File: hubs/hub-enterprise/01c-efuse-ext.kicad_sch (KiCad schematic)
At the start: 12 parts, among them J103 PJ-002AH, U103 TPS25940LRVCR

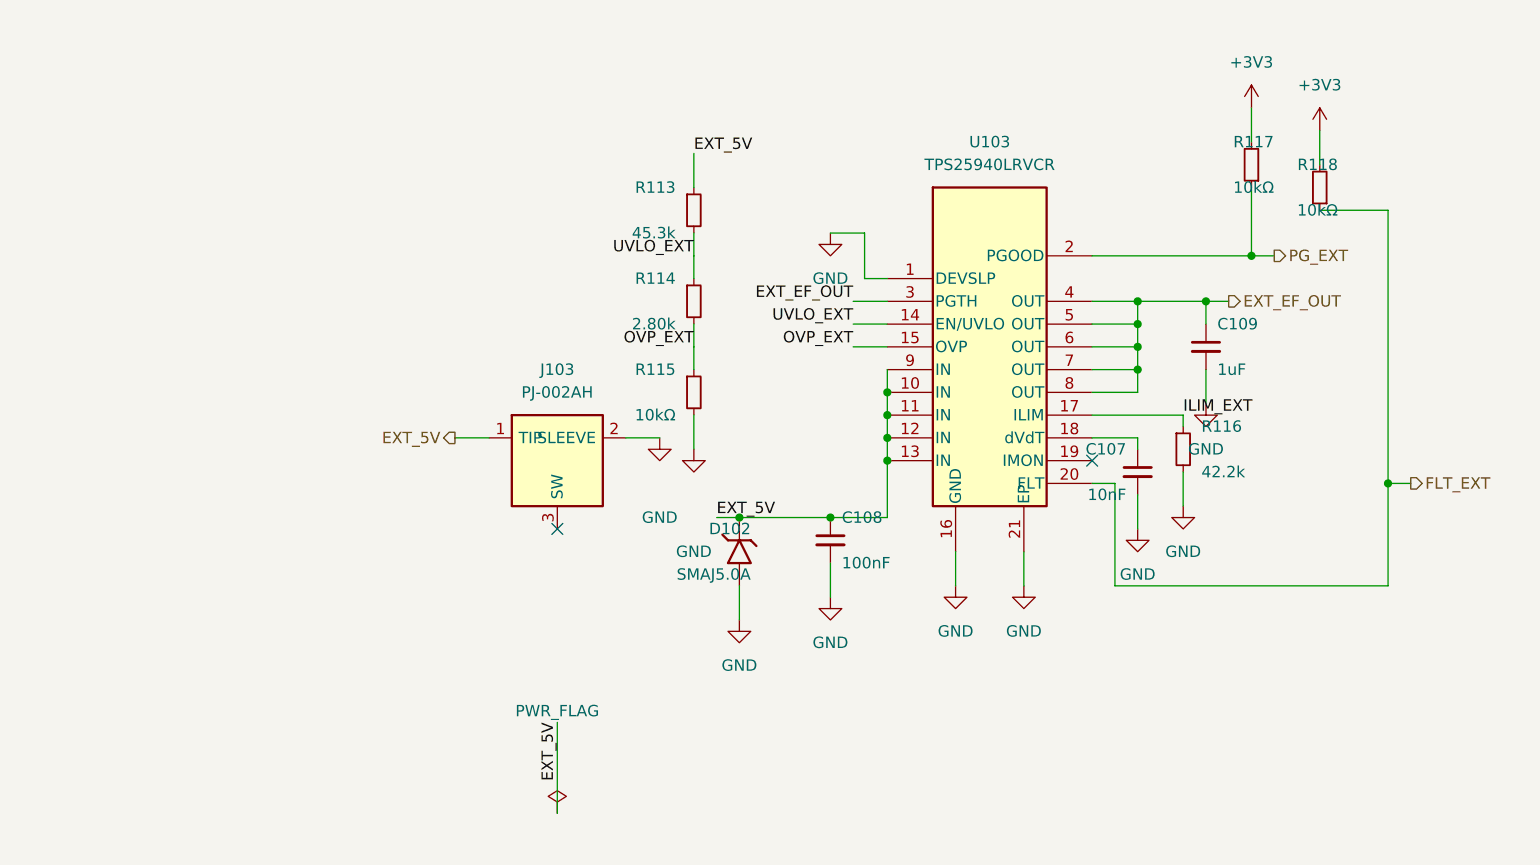
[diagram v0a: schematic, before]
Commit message: WIP snapshot: composition agent hub regeneration in flight (durability)
Co-Authored-By: Claude Fable 5 <noreply@anthropic.com>
Claude-Session: https://claude.ai/code/session_011q5bmwF5BFtSf8Ft5vT1DZ
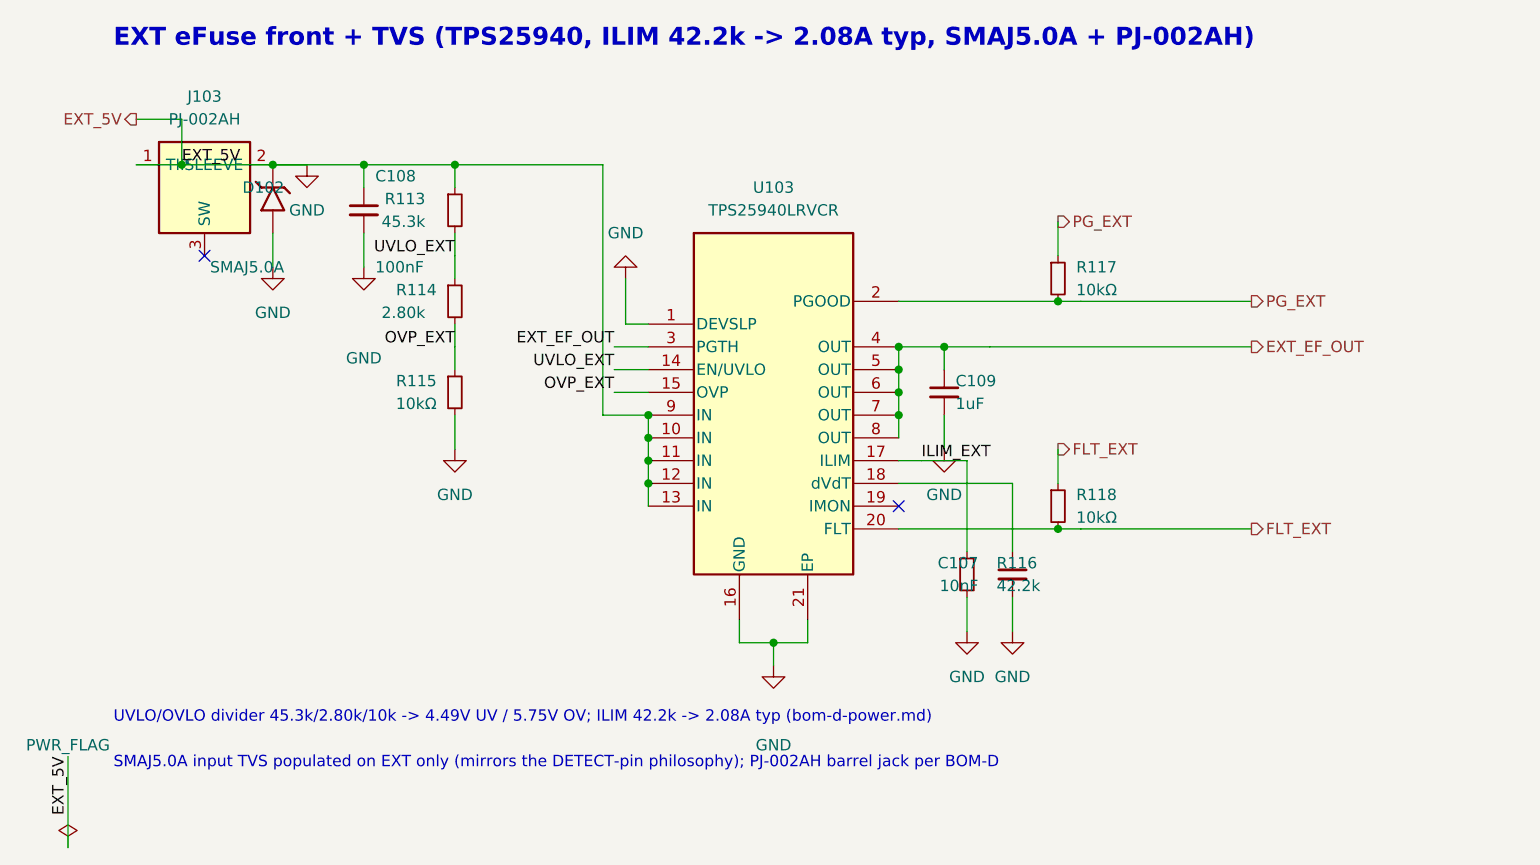
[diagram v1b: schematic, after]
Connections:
- net EXT_5V is gone; now on net GND: C108.1, D102.2 (K), J103.1 (TIP), R113.1, U103.10 (IN), U103.11 (IN), U103.12 (IN), U103.13 (IN), U103.9 (IN)
- net FLT_EXT: now also R118.2
- net PG_EXT: now also R117.2
- removed net +3V3: R117.2, R118.2
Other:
- note added: "EXT eFuse front + TVS (TPS25940, ILIM 42.2k -> 2.08A typ, SMAJ5.0A + PJ-002AH)"
- note added: "SMAJ5.0A input TVS populated on EXT only (mirrors the DETECT-pin philosophy); PJ-002AH barrel jack per BOM-D"
- note added: "UVLO/OVLO divider 45.3k/2.80k/10k -> 4.49V UV / 5.75V OV; ILIM 42.2k -> 2.08A typ (bom-d-power.md)"
